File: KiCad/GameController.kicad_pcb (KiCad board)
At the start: 2 copper layers, 152.4 x 61.9 mm, 14 parts, among them SW1 SW_Push, SW10 SW_Push, SW2 SW_Push, SW3 SW_Push, SW4 SW_Push, SW5 SW_Push, SW6 SW_Push, SW7 SW_Push, SW8 SW_Push, SW9 SW_Push, U1 COM-09032, U2 COM-09032, U3 MCP3008

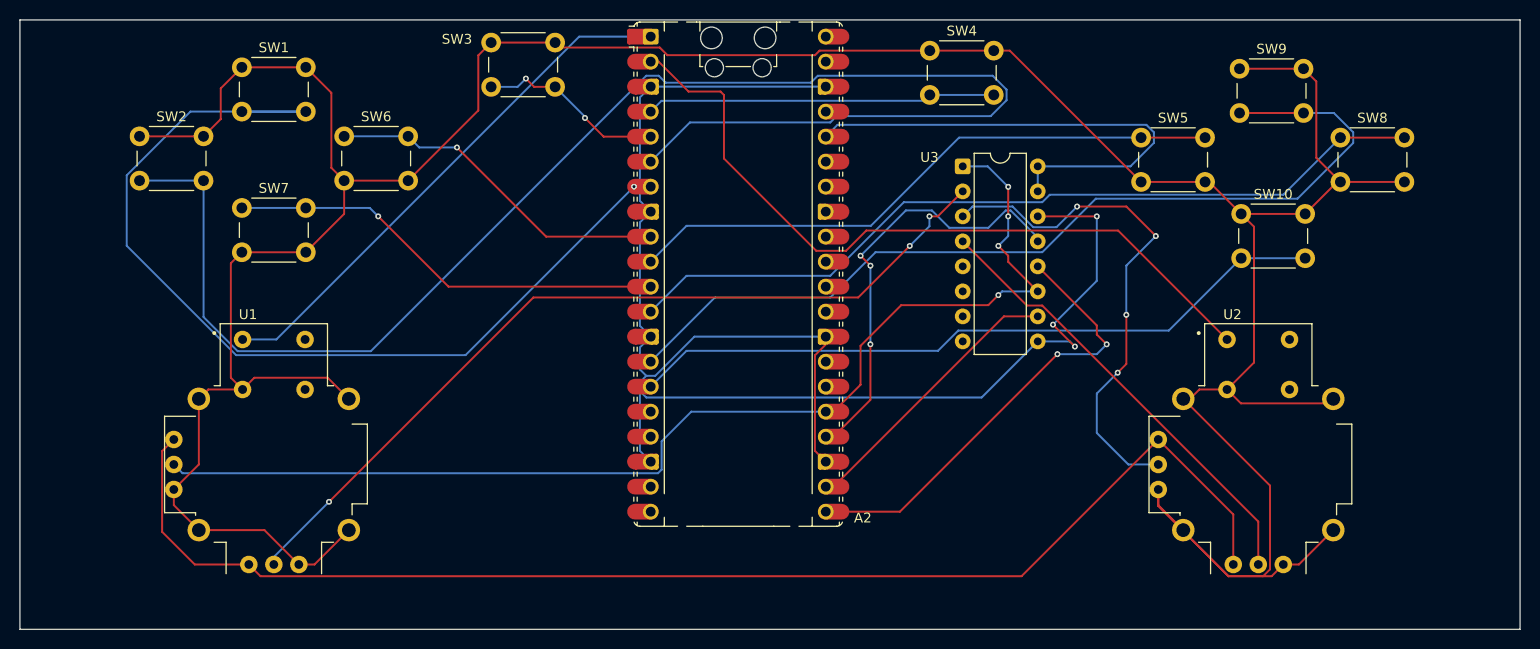
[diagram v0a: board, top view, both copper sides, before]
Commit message: UP
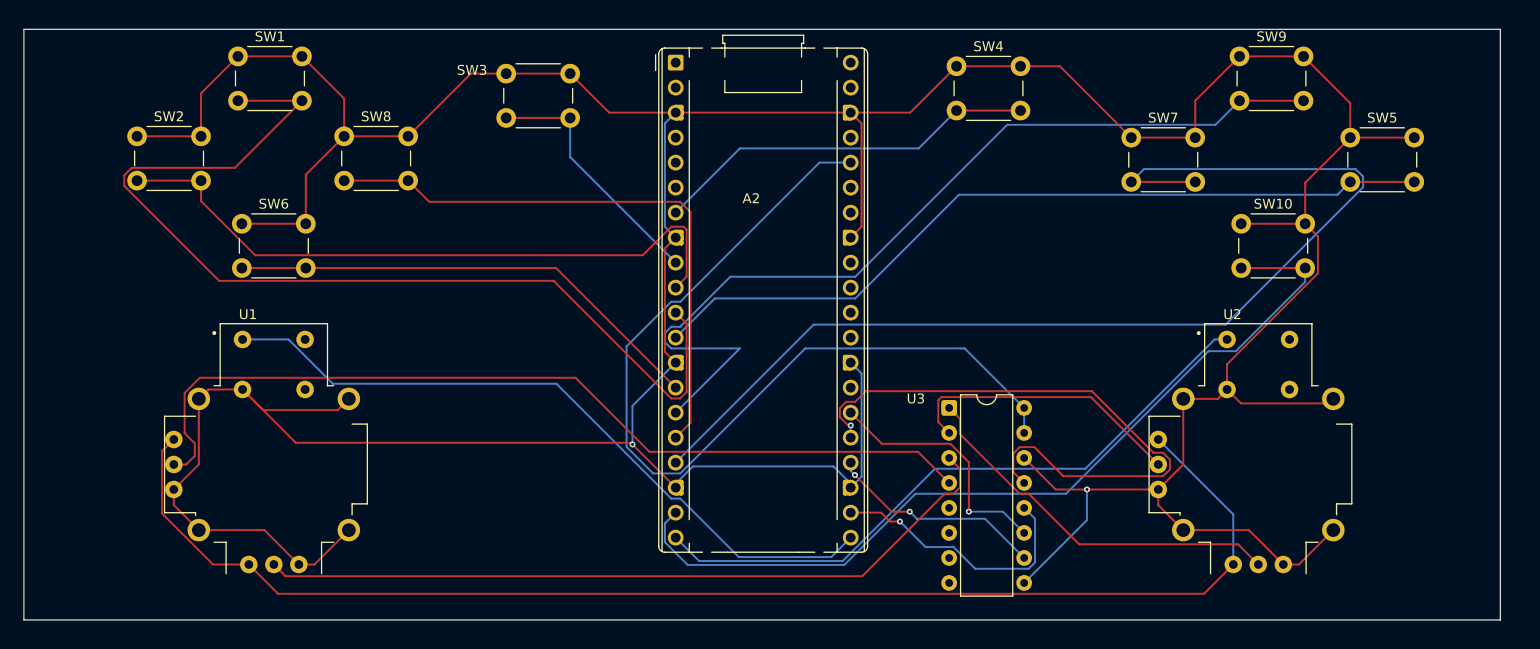
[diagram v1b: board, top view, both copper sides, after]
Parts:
- A2: footprint Module:RaspberryPi_Pico_Common_Unspecified -> Module:RaspberryPi_Pico_Common_THT
- moved U3 24.6 mm to (171.0, 120.5)
- moved A2 22.4 mm to (143.2, 85.4)
- moved SW3 3.51 mm to (126.0, 86.5)
- moved SW4 3.15 mm to (171.8, 85.8)
- moved SW6 1.61 mm to (99.1, 101.8)
- moved SW9 1.25 mm to (200.5, 84.8)
- moved SW1 1.17 mm to (98.8, 84.8)
- moved SW10 1.00 mm to (200.7, 101.8)
- moved SW5 1.00 mm to (211.8, 93.0)
- moved SW7 1.00 mm to (189.5, 93.0)
- moved SW2 0.25 mm to (88.5, 92.9)
- renumbered SW8 to SW5, SW7 to SW6, SW5 to SW7, SW6 to SW8
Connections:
- net Net-(A2-3V3) renamed /3V3
- A2 pad 1: Net-(A2-GPIO0) -> unconnected-(A2-GPIO0-Pad1)
- A2 pad 10: Net-(A2-GPIO7) -> /GPIO7
- A2 pad 11: Net-(A2-GPIO8) -> /GPIO8
- A2 pad 12: Net-(A2-GPIO9) -> /GPIO9
- A2 pad 13: Net-(U3-AGND) -> GND
- A2 pad 14: Net-(A2-GPIO10) -> /GPIO10
- A2 pad 15: Net-(A2-GPIO11) -> /GPIO11
- A2 pad 16: unconnected-(A2-GPIO12-Pad16) -> /GPIO12
- A2 pad 17: unconnected-(A2-GPIO13-Pad17) -> /GPIO13
- A2 pad 18: Net-(U3-AGND) -> GND
- A2 pad 19: unconnected-(A2-GPIO14-Pad19) -> /GPIO14
- A2 pad 2: Net-(A2-GPIO1) -> unconnected-(A2-GPIO1-Pad2)
- A2 pad 20: unconnected-(A2-GPIO15-Pad20) -> /GPIO15
- A2 pad 21: Net-(A2-GPIO16) -> /GPIO20
- A2 pad 22: Net-(A2-GPIO17) -> /GPIO19
- A2 pad 23: Net-(U3-AGND) -> GND
- A2 pad 24: Net-(A2-GPIO18) -> /GPIO18
- A2 pad 25: Net-(A2-GPIO19) -> /GPIO17
- A2 pad 26: unconnected-(A2-GPIO20-Pad26) -> /GPIO16
- A2 pad 28: Net-(U3-AGND) -> GND
- A2 pad 3: Net-(U3-AGND) -> GND
- A2 pad 33: unconnected-(A2-AGND-Pad33) -> GND
- A2 pad 38: Net-(U3-AGND) -> GND
- A2 pad 4: Net-(A2-GPIO2) -> unconnected-(A2-GPIO2-Pad4)
- A2 pad 5: Net-(A2-GPIO3) -> unconnected-(A2-GPIO3-Pad5)
- A2 pad 6: Net-(A2-GPIO4) -> unconnected-(A2-GPIO4-Pad6)
- A2 pad 7: Net-(A2-GPIO5) -> /GPIO5
- A2 pad 8: Net-(U3-AGND) -> GND
- A2 pad 9: Net-(A2-GPIO6) -> /GPIO6
- SW1 pad 2: Net-(A2-GPIO5) -> /GPIO8
- SW10 pad 2: Net-(A2-GPIO11) -> /GPIO14
- SW2 pad 2: Net-(A2-GPIO4) -> /GPIO7
- SW3 pad 2: Net-(A2-GPIO3) -> /GPIO6
- SW4 pad 2: Net-(A2-GPIO2) -> /GPIO5
- SW5 pad 1: Net-(A2-GPIO9) -> GND
- SW5 pad 2: GND -> /GPIO9
- SW6 pad 1: Net-(A2-GPIO8) -> GND
- SW6 pad 2: GND -> /GPIO10
- SW7 pad 1: Net-(A2-GPIO7) -> GND
- SW7 pad 2: GND -> /GPIO13
- SW8 pad 1: Net-(A2-GPIO6) -> GND
- SW8 pad 2: GND -> /GPIO12
- SW9 pad 2: Net-(A2-GPIO10) -> /GPIO11
- U1 pad B1A: Net-(A2-GPIO0) -> /GPIO20
- U1 pad H2: Net-(U1-H) -> /CH1
- U1 pad V2: Net-(A2-GPIO19) -> /CH0
- U2 pad B1A: Net-(A2-GPIO1) -> /GPIO15
- U2 pad H2: Net-(U2-H) -> /CH3
- U2 pad V2: Net-(U2-V) -> /CH2
- U3 pad 1: Net-(A2-GPIO19) -> /CH3
- U3 pad 10: Net-(A2-GPIO17) -> /GPIO18
- U3 pad 11: Net-(A2-GPIO19) -> /GPIO16
- U3 pad 12: Net-(A2-GPIO16) -> /GPIO19
- U3 pad 13: Net-(A2-GPIO18) -> /GPIO17
- U3 pad 14: Net-(U3-AGND) -> GND
- U3 pad 2: Net-(U1-H) -> /CH2
- U3 pad 3: Net-(U2-V) -> /CH1
- U3 pad 4: Net-(U2-H) -> /CH0
- U3 pad 9: Net-(U3-AGND) -> GND
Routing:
- net Net-(U3-AGND): track 162.9 -> 0.00 mm, vias 3 -> 0
- net Net-(A2-GPIO4): track 155.9 -> 0.00 mm
- net GND: track 358.4 -> 478.0 mm, vias 0 -> 2
- net Net-(A2-GPIO19): track 117.2 -> 0.00 mm, vias 4 -> 0
- net /GPIO13: track 0.00 -> 113.4 mm
- net /GPIO8: track 0.00 -> 103.6 mm
- net Net-(A2-GPIO10): track 100.5 -> 0.00 mm
- net Net-(A2-GPIO5): track 99.5 -> 0.00 mm, vias 1 -> 0
- net /GPIO11: track 0.00 -> 92.7 mm
- net /CH0: track 0.00 -> 92.1 mm
- net /GPIO14: track 0.00 -> 89.3 mm
- net Net-(U1-H): track 86.7 -> 0.00 mm, vias 3 -> 0
- net Net-(A2-GPIO9): track 83.9 -> 0.00 mm
- net /GPIO9: track 0.00 -> 81.6 mm
- net /CH1: track 0.00 -> 77.4 mm
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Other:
- board size 152.4 x 61.9 mm -> 150 x 60 mm
